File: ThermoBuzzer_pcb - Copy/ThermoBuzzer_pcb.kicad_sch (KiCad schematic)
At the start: 10 parts, among them SW2 SW_Push

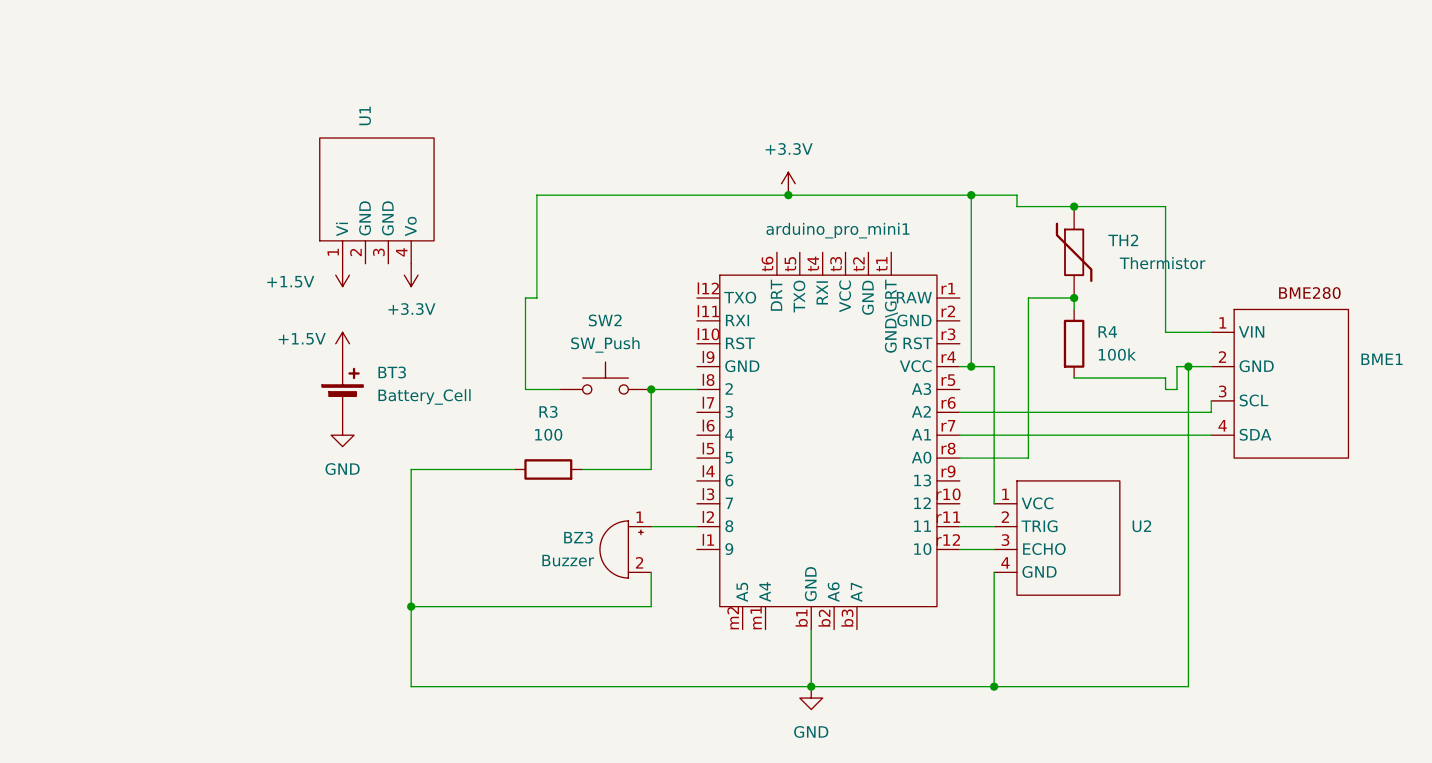
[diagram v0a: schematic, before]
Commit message: 4.21
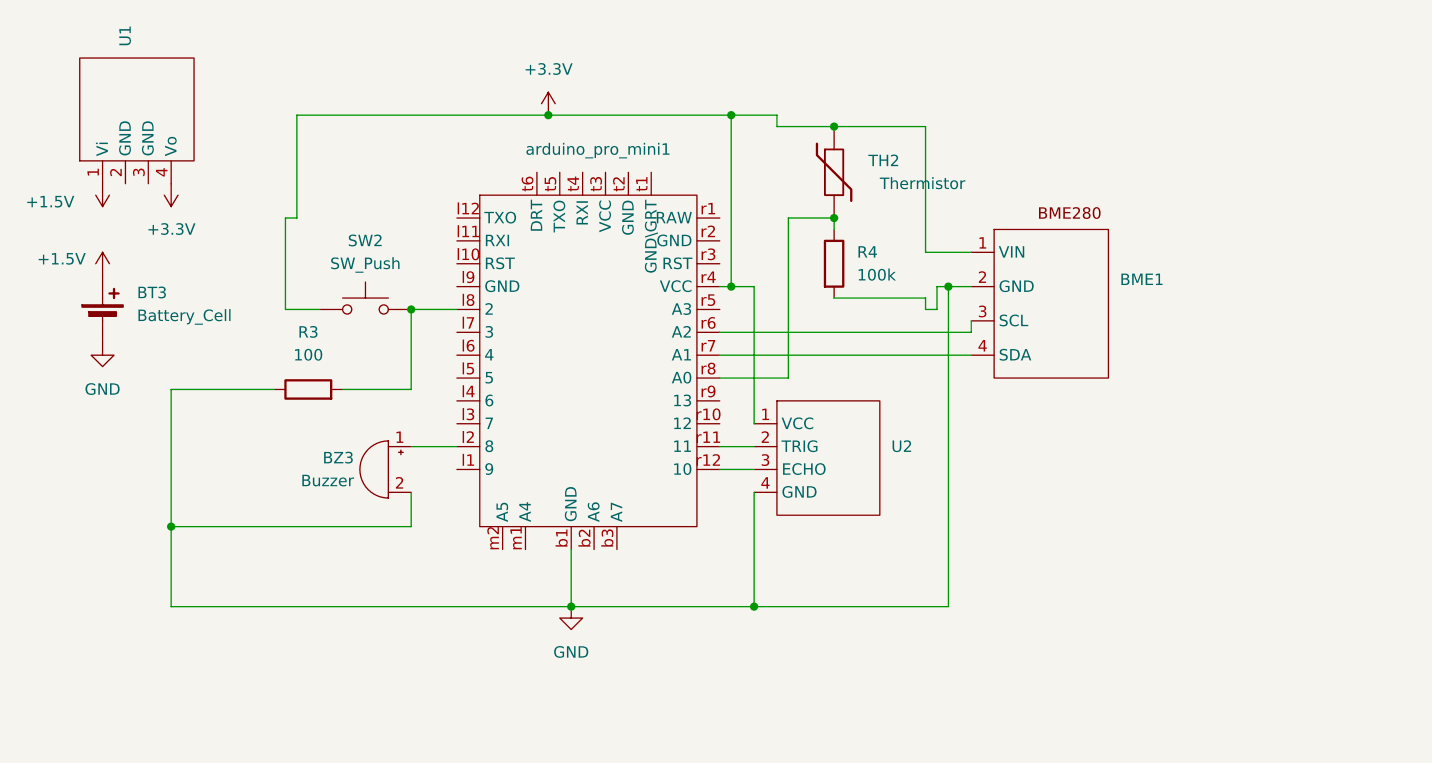
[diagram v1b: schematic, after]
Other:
- moved on the sheet: BME1, BT3, BZ3, R3, R4, SW2, TH2, U1, U2, arduino_pro_mini1
